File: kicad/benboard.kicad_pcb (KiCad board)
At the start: 4 copper layers, 140 x 88.4 mm, 111 parts, among them J1 USB_C_Receptacle_USB2.0, J3 Conn_ARM_SWD_TagConnect_TC203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, J4 Conn_01x02_Pin, J5 Conn_Coaxial, SW1 SW_Push, SW10 SW_Push, SW11 SW_Push, SW12 SW_Push, SW13 SW_Push, SW14 SW_Push, SW15 SW_Push, SW16 SW_Push, SW17 SW_Push, SW18 SW_Push, SW19 SW_Push, SW2 SW_Push, SW20 SW_Push, SW21 SW_Push, SW22 SW_DPDT, SW3 SW_Push, SW4 SW_Push, SW5 SW_Push, SW6 SW_Push, SW7 SW_Push, SW8 SW_Push, SW9 SW_Push, U1 nRF52840, U2 TPS61222DCK, U3 nPM1300-QEXX, Y1 32MHz, Y2 32.768kHz

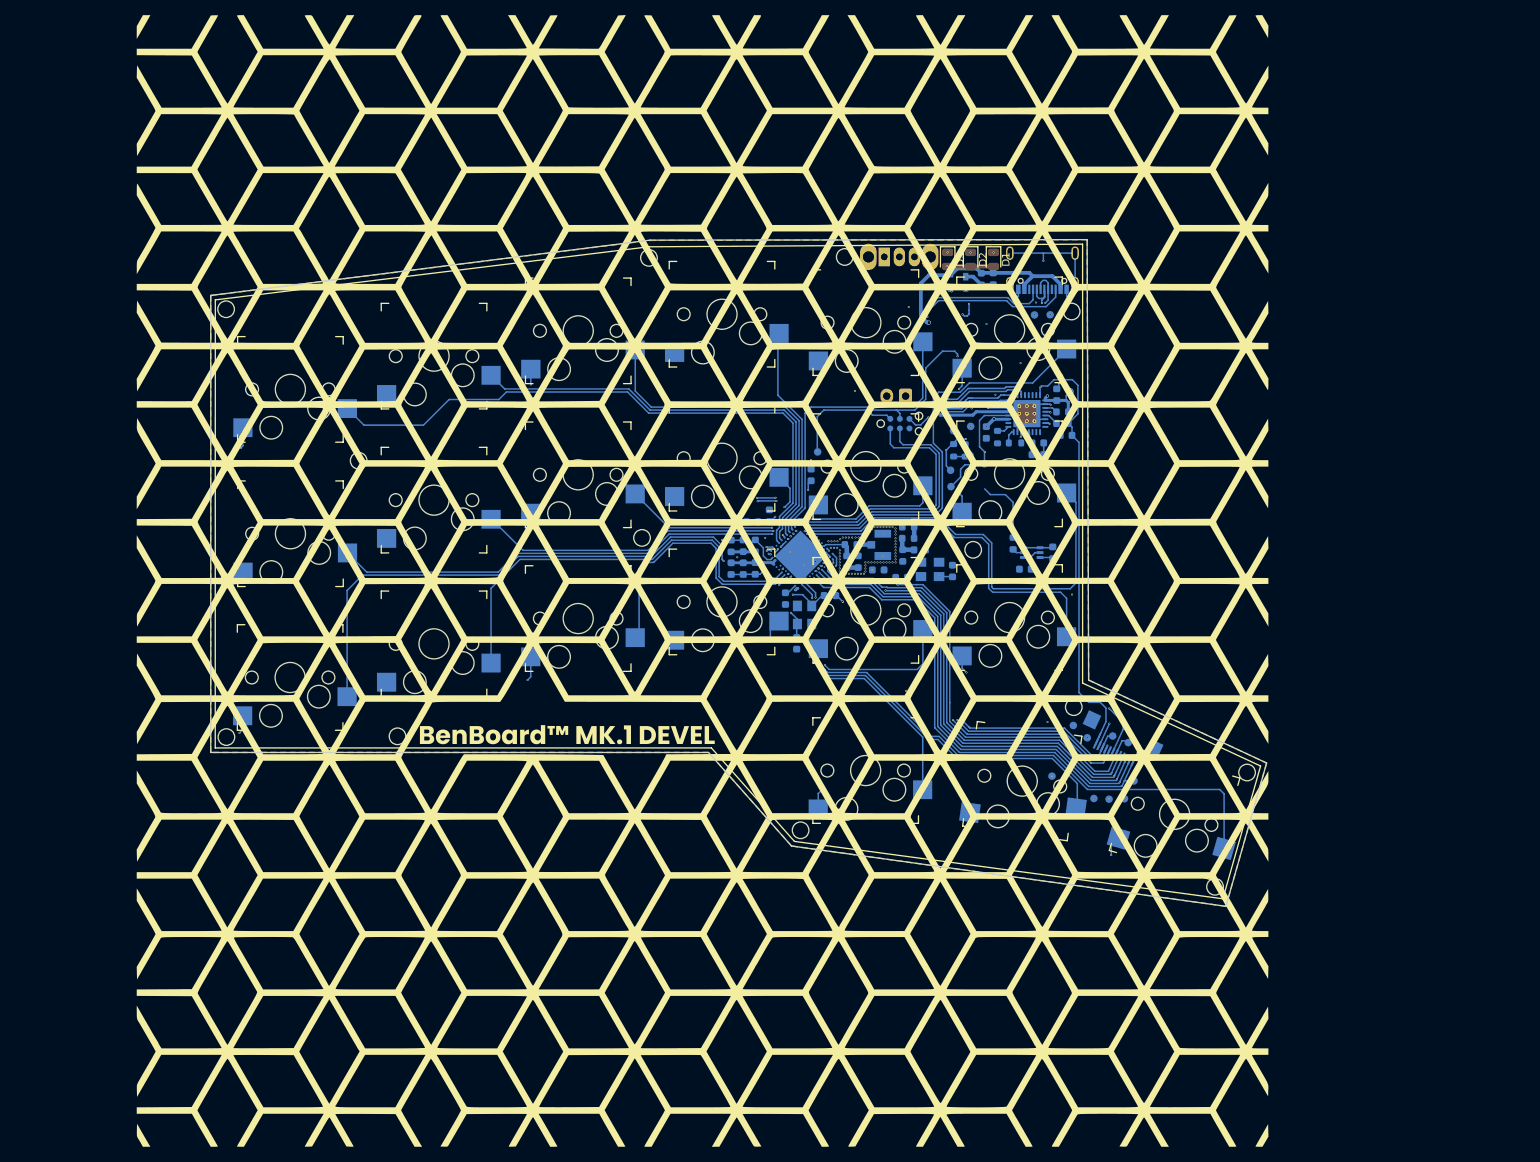
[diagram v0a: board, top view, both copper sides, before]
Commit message: new revision
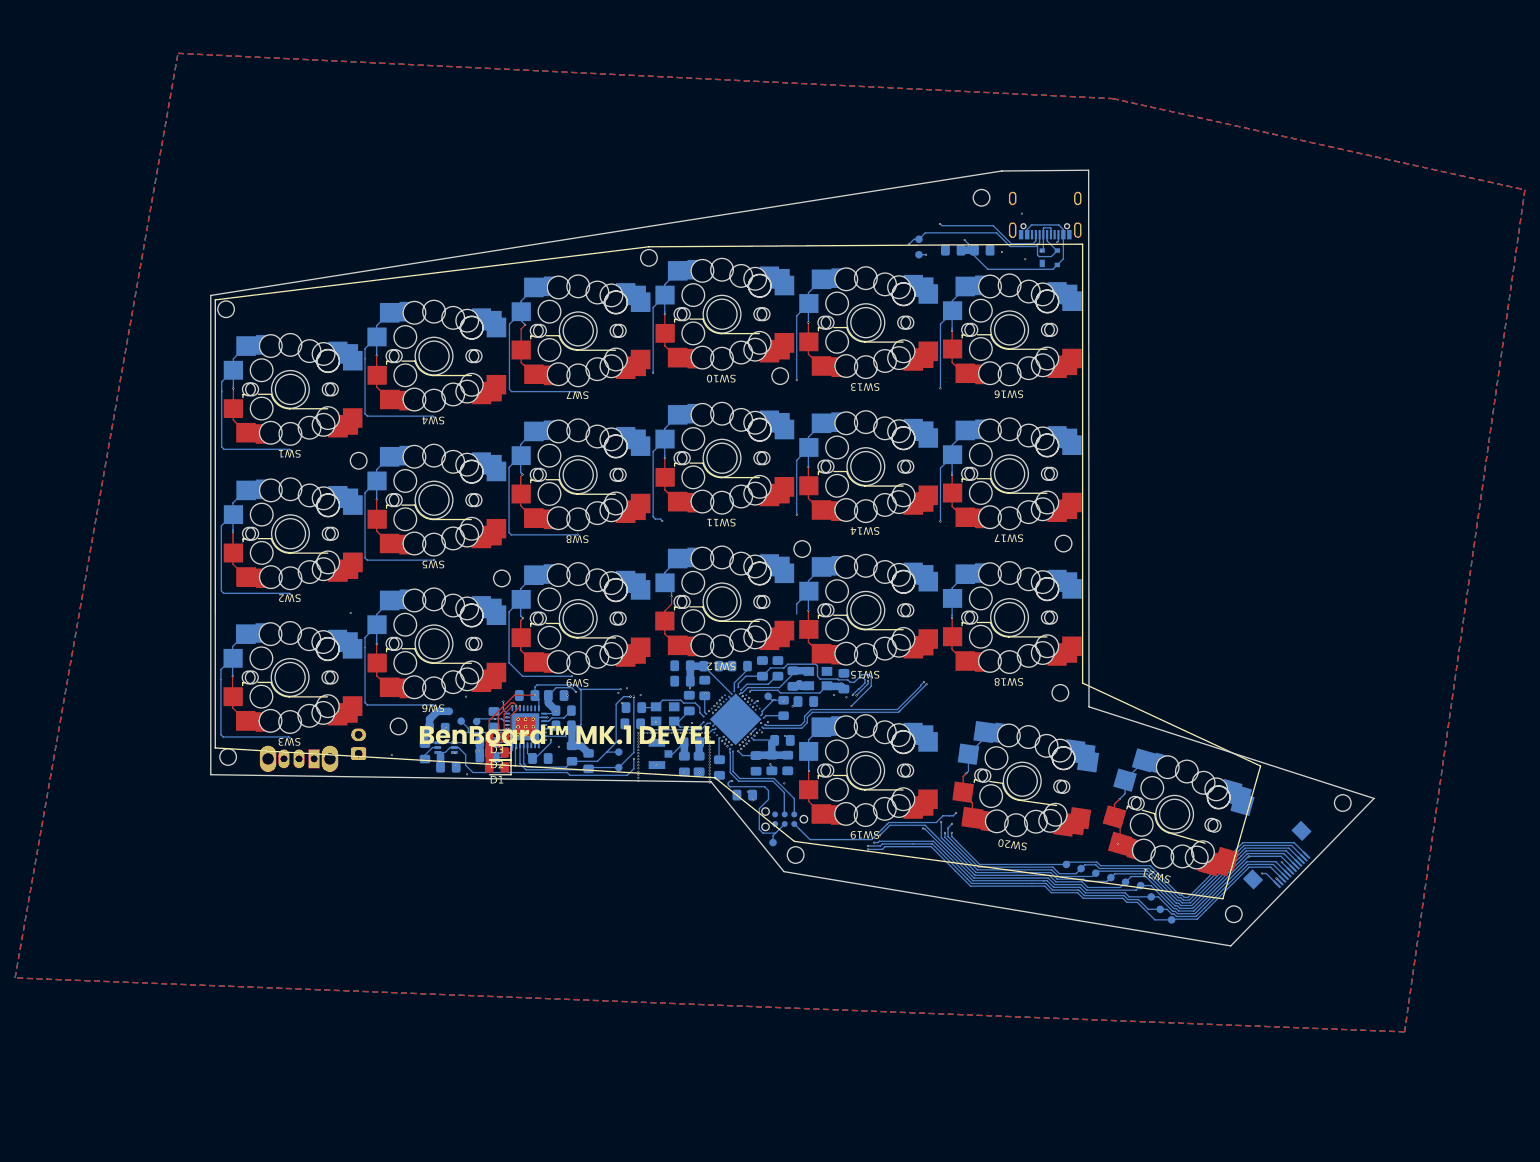
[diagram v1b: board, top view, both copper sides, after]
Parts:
- removed the G*** at (127.4, 88.3)
- removed the REF** at (176.6, 105.0)
- removed the REF** at (146.3, 45.3)
- added ?: , , F.Cu at (137.7, 61.1)
- added ?: , , F.Cu at (100.8, 87.9)
- added ?: , , F.Cu at (212.3, 117.7)
- C1, C10, C11, C12, C13, C14, C15, C16, C17, C18, C19, C2, C20, C21, C22, C23, C24, C25, C26, C27, C3, C4, C5, C6, C7, C8, C9: footprint Capacitor_SMD:C_0603_1608Metric -> Capacitor_SMD:C_0805_2012Metric_Pad1.18x1.45mm_HandSolder
- D1, D2, D3: footprint LED_SMD:LED_0805_2012Metric -> LED_SMD:LED_0805_2012Metric_Pad1.15x1.40mm_HandSolder
- L1, L2, L3, L4, L5, L6, L7: footprint Inductor_SMD:L_0603_1608Metric -> Inductor_SMD:L_0805_2012Metric_Pad1.15x1.40mm_HandSolder
- R1, R2, R3, R4: footprint Resistor_SMD:R_0603_1608Metric -> Inductor_SMD:L_0805_2012Metric_Pad1.15x1.40mm_HandSolder
- SW1, SW10, SW11, SW12, SW13, SW14, SW15, SW16, SW17, SW18, SW19, SW2, SW20, SW21, SW3, SW4, SW5, SW6, SW7, SW8, SW9: footprint keyswitches:Kailh_socket_MX -> fingerpunch:gateron-ks27-choc-v1-mx-hotswap-reversible
- moved SW22 100.7 mm to (75.9, 111.8), turned to 180 degrees
- moved D1 94.2 mm to (100.2, 113.0), turned to 180 degrees
- moved D2 90.6 mm to (100.2, 111.0), turned to 180 degrees
- moved D3 87.1 mm to (100.2, 109.0), turned to 180 degrees
- moved J4 86.6 mm to (81.8, 111.2), turned to 90 degrees
- moved C18 84.8 mm to (92.2, 107.8), turned to 0 degrees
- moved L5 82.7 mm to (90.6, 110.8)
- moved U2 81.8 mm to (93.4, 110.3)
- moved R2 81.4 mm to (98.9, 111.7), turned to 0 degrees
- moved C19 80.9 mm to (93.7, 113.0), turned to 0 degrees
- moved C25 79.4 mm to (104.2, 103.5)
- moved R1 78.8 mm to (98.9, 109.7), turned to 180 degrees
- moved U3 78.4 mm to (104.0, 107.6)
- moved TP15 78.2 mm to (93.8, 105.5)
- moved C26 78.1 mm to (105.9, 111.8)
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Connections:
- U1 pad AC17: SW5 -> SW9
- U1 pad AC19: SW8 -> SW6
- U1 pad AC21: SW11 -> SW3
- U1 pad AD10: SW1 -> SW4
- U1 pad AD12: SW4 -> SW7
- U1 pad AD16: SW7 -> SW10
- U1 pad AD18: SW10 -> SW13
- U1 pad AD20: SW13 -> SW16
- U1 pad AD22: SW14 -> SW11
- U1 pad H2: SW12 -> SW18
- U1 pad L1: SW9 -> SW1
- U1 pad N1: SW6 -> SW8
- U1 pad P2: SW3 -> SW5
- U1 pad P23: SW15 -> SW19
- U1 pad R24: SW18 -> SW12
- U1 pad T23: SW21 -> SW20
- U1 pad V23: SW20 -> SW21
- U1 pad W24: SW16 -> SW14
- U1 pad Y23: SW19 -> SW15
- U3 pad 18: Net-(U3-NTC) -> GND
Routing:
- net +5V: track 37.7 -> 152.8 mm, vias 2 -> 3
- net VBUS_IN: track 51.2 -> 151.3 mm
- net CC2: track 42.4 -> 134.8 mm
- net CC1: track 40.9 -> 131.2 mm
- net SW16: track 54.4 -> 138.8 mm, vias 0 -> 3
- net SW14: track 20.9 -> 103.6 mm, vias 0 -> 3
- net SW11: track 8.98 -> 87.4 mm, vias 2 -> 3
- net SW13: track 40.1 -> 116.9 mm, vias 0 -> 3
- net SW4: track 59.7 -> 135.6 mm, vias 0 -> 3
- net SW10: track 28.6 -> 99.8 mm, vias 0 -> 3
- net SW7: track 44.8 -> 115.0 mm, vias 0 -> 3
- net SW17: track 56.0 -> 123.4 mm, vias 0 -> 3
- net VBAT: track 71.9 -> 10.1 mm, vias 3 -> 0
- net GND: track 85.0 -> 24.5 mm, vias 109 -> 85
- net SW12: track 13.5 -> 72.0 mm
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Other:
- board size 140 x 88.4 mm -> 154.2 x 102.9 mm
